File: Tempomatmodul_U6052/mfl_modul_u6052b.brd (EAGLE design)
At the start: 78 x 58 mm, 27 parts, among them IC1 U6052B-A, J1 43045-0800, K1 APF30212C, K2 APF30212C, K3 APF30212C, K4 APF30212C

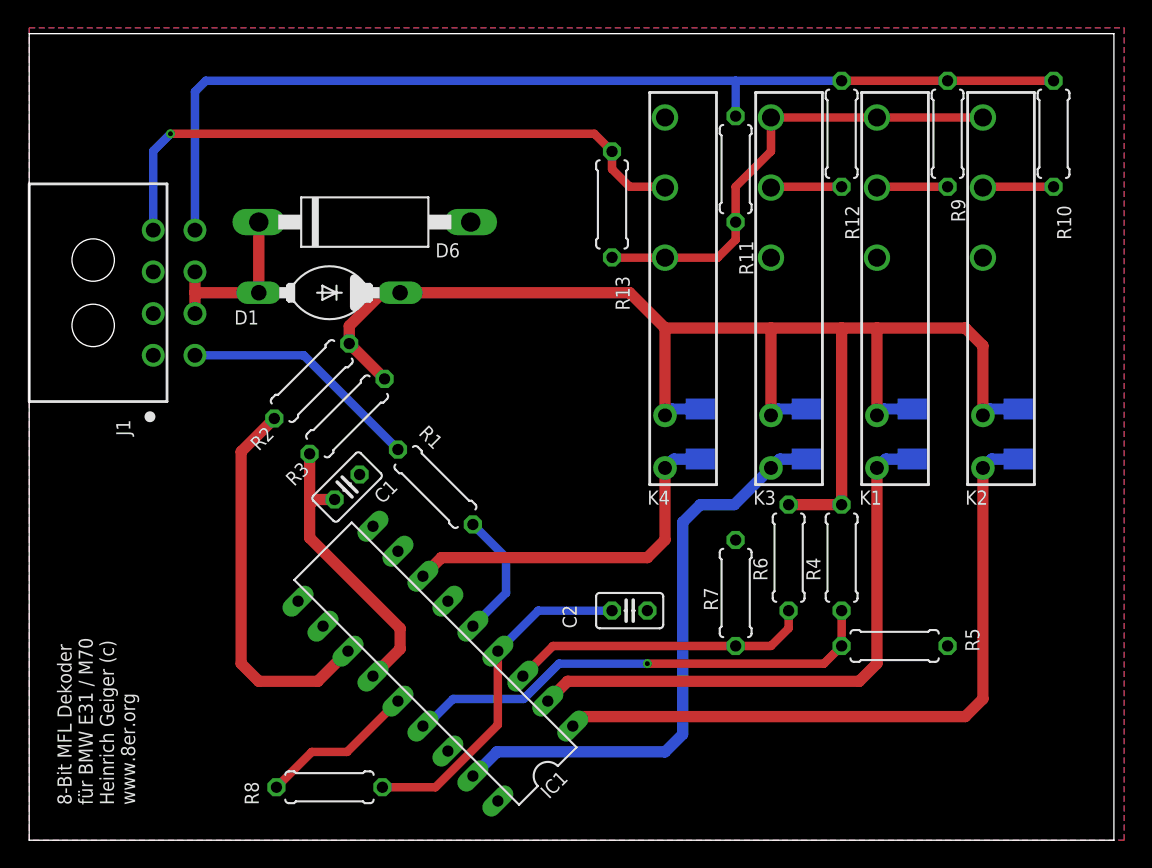
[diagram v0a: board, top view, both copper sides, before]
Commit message: Fixed. Running version!
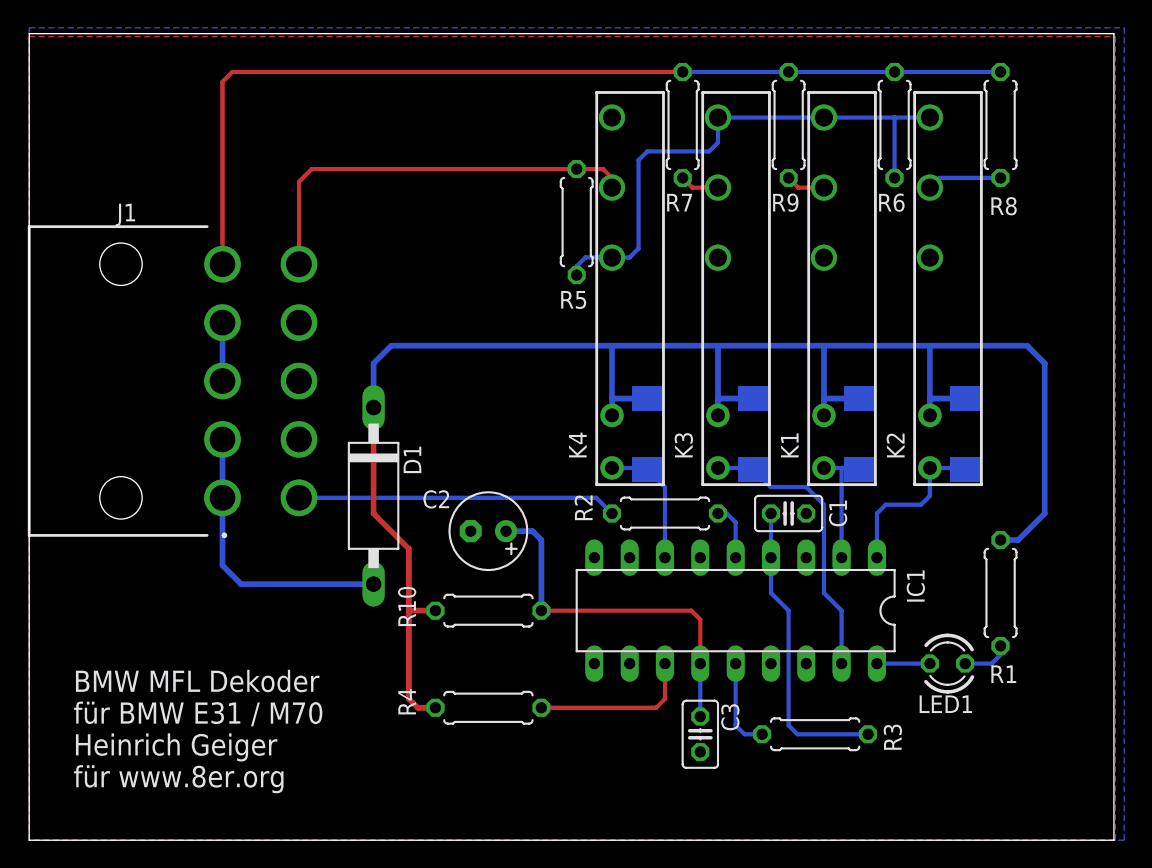
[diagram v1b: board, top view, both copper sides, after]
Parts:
- removed D6: P6KEXXC, diode:CB417-15
- removed R11, R12: 665, rcl:0207/7
- removed R13: 931, rcl:0207/7
- added C3: 100nF, rcl:C025-025X050
- added LED1: led grün 2,2v 20mA, led:LED3MM
- C1: value 100µF -> 1nF
- C2: value 1nF -> 100uF/36V; device rcl:C025-025X050 -> rcl:E2,5-6
- D1: value BYW52 -> EP20D; device diode:DO204-10 -> diode:DO15-12
- D2, D3, D4, D5: value CGRM4004-G -> MBSR140; device diode:SOD-123_MINI-SMA -> Heinrich:DO214AA
- J1: value 43045-0800 -> 39-30-1100; device Heinrich:43045-0800 -> Heinrich:39-30-1100
- R1: value 100 -> 560
- R10: value 200 -> 510
- R2: value 510 -> 100
- R3: value 200 -> 200k
- R4: value 270k -> 200
- R5: value 20k -> 931
- R6: value 150k -> 665
- R7: value 39k -> 665
- R8: value 200k -> 200
- R9: value 66.5 -> 66,5
- moved R8 67.8 mm to (69.8, 51.4), turned to 90 degrees
- moved R10 53.2 mm to (33.0, 16.5), turned to 0 degrees
- moved R3 44.2 mm to (56.5, 7.62), turned to 0 degrees
- moved R1 41.3 mm to (69.8, 17.8), turned to 90 degrees
- moved R5 38.1 mm to (39.4, 44.5), turned to 270 degrees
- moved R7 33.9 mm to (47.0, 51.4), turned to 90 degrees
- moved R6 32.0 mm to (62.2, 51.4), turned to 90 degrees
- moved C1 31.8 mm to (54.6, 23.5), turned to 0 degrees
- moved R4 27.6 mm to (33.0, 9.53), turned to 0 degrees
- moved R2 23.9 mm to (45.7, 23.5), turned to 0 degrees
- moved IC1 21.9 mm to (50.8, 16.5), turned to 180 degrees
- moved D1 14.9 mm to (24.8, 24.8), turned to 270 degrees
- moved C2 11.7 mm to (33.0, 22.2), turned to 180 degrees
- moved R9 11.4 mm to (54.6, 51.4)
- moved J1 6.35 mm to (0.00, 33.0)
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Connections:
- net K1 renamed PLUS
- net K2 renamed ABRUF
- net K3 renamed MINUS
- net K4 renamed I/O
- removed net +12V: D1.C, D2.C, D3.C, D4.C, D5.C, K1.2, K2.2, K3.2, K4.2, R2.1, R3.1, R4.1, R6.1
- removed net LD: IC1.15, R4.2, R5.2
- removed net MFL_CC: J1.5, R1.1
- removed net N$6: K1.NO, K2.NO, K3.NO, K4.NC, R11.1, R13.2
- removed net N$8: K2.COM, R10.1
- removed net PO: IC1.3, R6.2, R7.2
- new net IBUS: J1.3, J1.4
- new net MFL: J1.6, R2.1
- new net N$10: K2.COM, R8.1
- new net N$11: K3.COM, R7.1
- new net N$12: K1.NO, K2.NO, K3.NO, K4.NC, R5.2, R6.1
- new net N$3: LED1.A, R1.1
- new net VCC: D1.C, D2.C, D3.C, D4.C, D5.C, K1.2, K2.2, K3.2, K4.2, R1.2, R10.1, R4.1
- net EML1: now also J1.5, R6.2, R7.2, R8.2; no longer J1.8, R10.2, R11.2, R12.2
- net EML2: now also J1.10, R5.1; no longer J1.4, R13.1
- net GND: now also C2.-, C3.2, IC1.15, IC1.3, J1.7, J1.8, J1.9; no longer C2.2, D6.A, J1.2, J1.3, R5.1, R7.1
- net N$1: now also R2.2; no longer R1.2
- net N$2: now also R4.2; no longer R3.2
- net N$4: now also IC1.18, LED1.K; no longer K3.COM, R12.1
- net OSC: now also C1.1, R3.2; no longer C2.1, R8.2
- net VBAT: now also J1.1, J1.2; no longer D6.C, J1.6, J1.7
- net VS: now also C2.+, C3.1, R10.2; no longer C1.1, R2.2
- net VSTAB: now also R3.1; no longer R8.1
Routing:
- net VCC: track 0.00 -> 123.5 mm
- net +12V: track 104.3 -> 0.00 mm
- net N$12: track 0.00 -> 39.6 mm
- net ABRUF: track 49.7 -> 12.1 mm
- net LD: track 35.0 -> 0.00 mm, vias 1 -> 0
- net N$6: track 34.5 -> 0.00 mm
- net PLUS: track 41.7 -> 9.04 mm
- net MFL: track 0.00 -> 23.0 mm
- net PO: track 21.8 -> 0.00 mm
- net MINUS: track 42.3 -> 20.7 mm
- net MFL_CC: track 17.4 -> 0.00 mm
- net I/O: track 26.5 -> 9.45 mm
- net N$2: track 27.7 -> 11.7 mm
- net EML2: track 45.4 -> 29.8 mm, vias 1 -> 0
- net VBAT: track 12.7 -> 20.5 mm
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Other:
- board text added: "BMW MFL Dekoder für BMW E31 / M70 Heinrich Geiger für www.8er.org"
- board text removed: "8-Bit MFL Dekoder für BMW E31 / M70 Heinrich Geiger (c) www.8er.org"
